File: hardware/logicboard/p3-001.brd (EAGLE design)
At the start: 42 x 83 mm, 28 parts, among them IC1 74LS07N, IC2 LTC485N, IC3 LTC485N

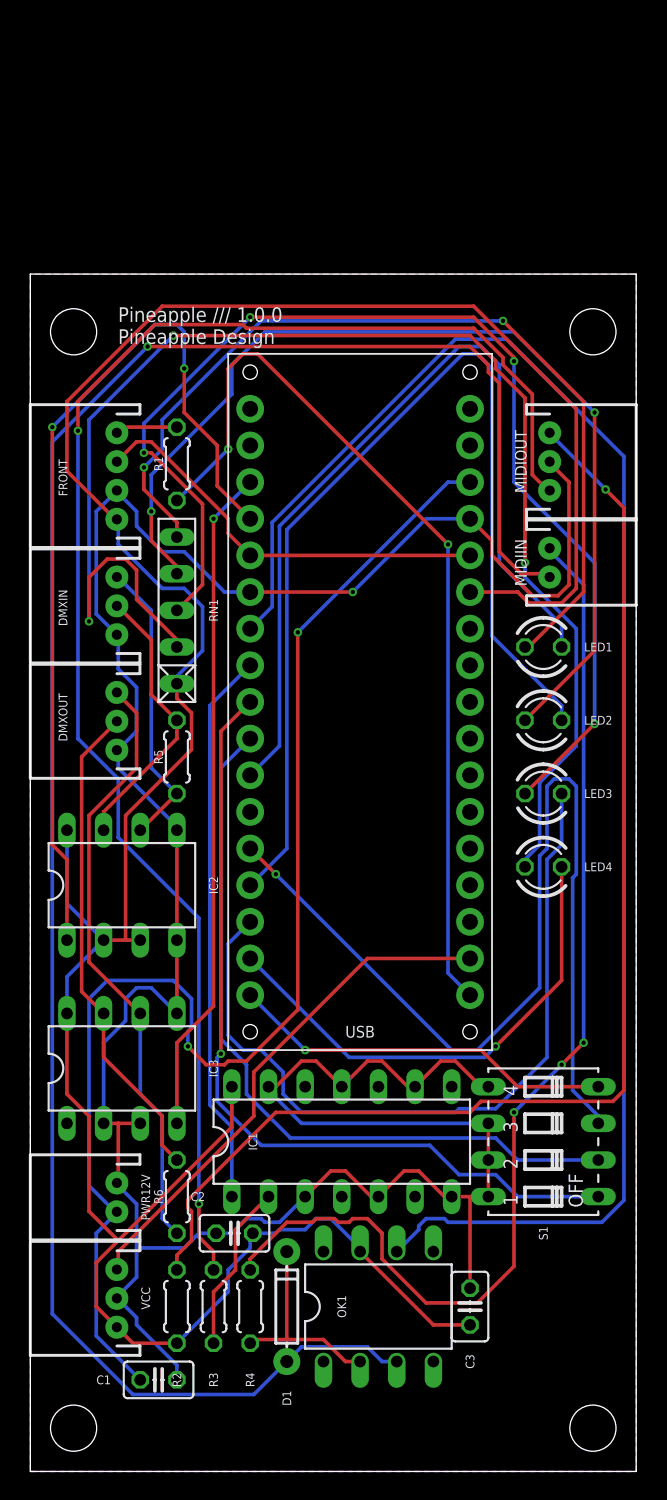
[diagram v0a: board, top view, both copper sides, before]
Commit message: 100mm board.
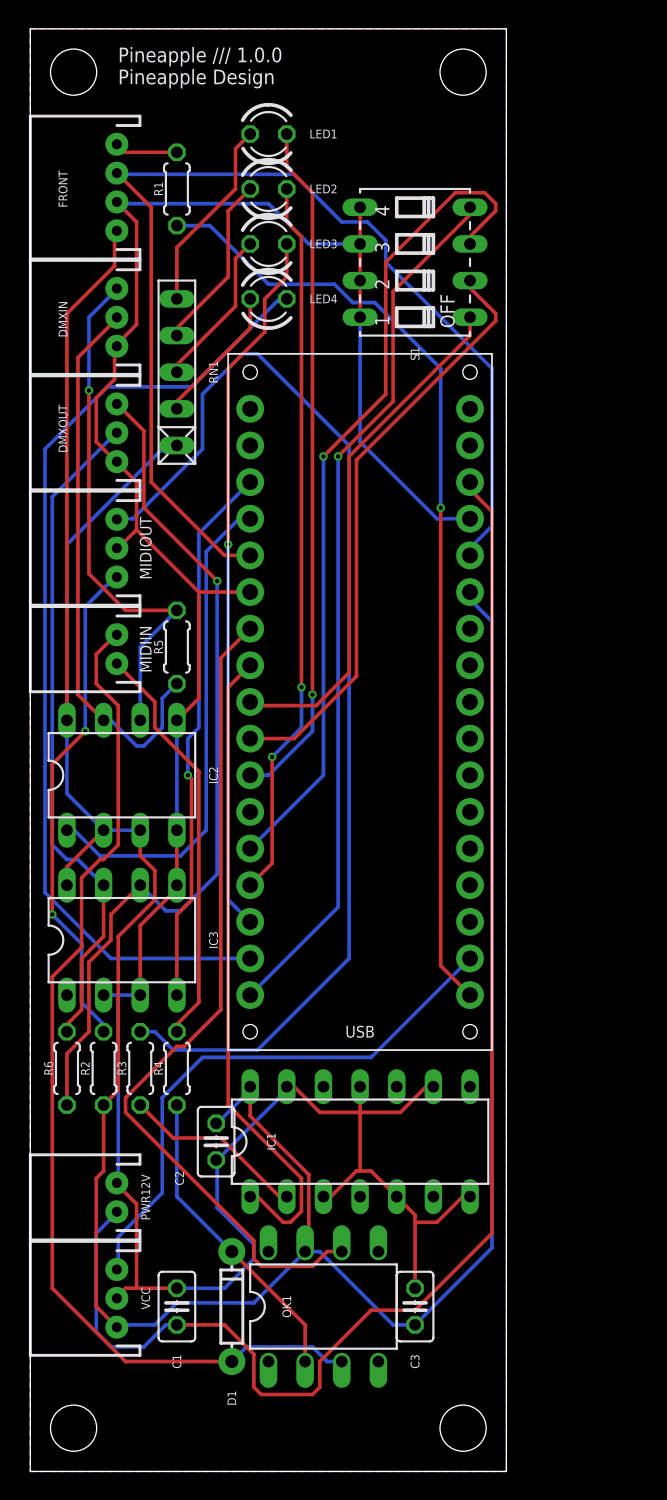
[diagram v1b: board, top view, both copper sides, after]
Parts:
- moved S1 61.6 mm to (26.7, 83.8)
- moved LED4 43.7 mm to (16.5, 81.3)
- moved LED3 42.6 mm to (16.5, 85.1)
- moved LED2 41.5 mm to (16.5, 88.9)
- moved LED1 40.3 mm to (16.5, 92.7)
- moved MIDIIN 30.6 mm to (6.00, 57.0), turned to 90 degrees
- moved MIDIOUT 30.6 mm to (6.00, 64.0), turned to 90 degrees
- moved DMXIN 20.0 mm to (6.00, 80.0)
- moved DMXOUT 20.0 mm to (6.00, 72.0)
- moved FRONT 20.0 mm to (6.00, 89.0)
- moved R1 19.1 mm to (10.2, 88.9)
- moved R2 17.3 mm to (5.08, 27.9)
- moved R3 17.3 mm to (7.62, 27.9)
- moved R4 17.3 mm to (10.2, 27.9)
- moved RN1 16.5 mm to (10.2, 76.2)
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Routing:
- net N$18: track 97.8 -> 9.72 mm, vias 3 -> 0
- net N$17: track 80.1 -> 11.0 mm, vias 4 -> 0
- net MIDIIN-: track 139.4 -> 71.6 mm, vias 1 -> 0
- net N$16: track 69.3 -> 12.3 mm, vias 2 -> 0
- net RX: track 110.2 -> 58.0 mm
- net MIDITHRU+: track 86.4 -> 34.9 mm, vias 1 -> 2
- net N$15: track 62.8 -> 13.5 mm, vias 2 -> 0
- net MIDIIN+: track 77.7 -> 28.5 mm, vias 3 -> 0
- net RST: track 28.9 -> 77.5 mm
- net N$22: track 26.8 -> 60.9 mm
- net N$14: track 34.5 -> 67.9 mm, vias 1 -> 0
- net N$10: track 63.1 -> 34.4 mm, vias 2 -> 0
- net MIDITHRU-: track 107.3 -> 78.9 mm, vias 2 -> 0
- net N$19: track 57.8 -> 36.0 mm, vias 1 -> 0
- net N$12: track 71.8 -> 50.2 mm, vias 0 -> 2
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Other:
- board size 42 x 83 mm -> 33 x 100 mm
